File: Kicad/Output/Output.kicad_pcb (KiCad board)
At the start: 2 copper layers, 13 parts, among them J1 Conn_01x02, J2 Conn_01x03

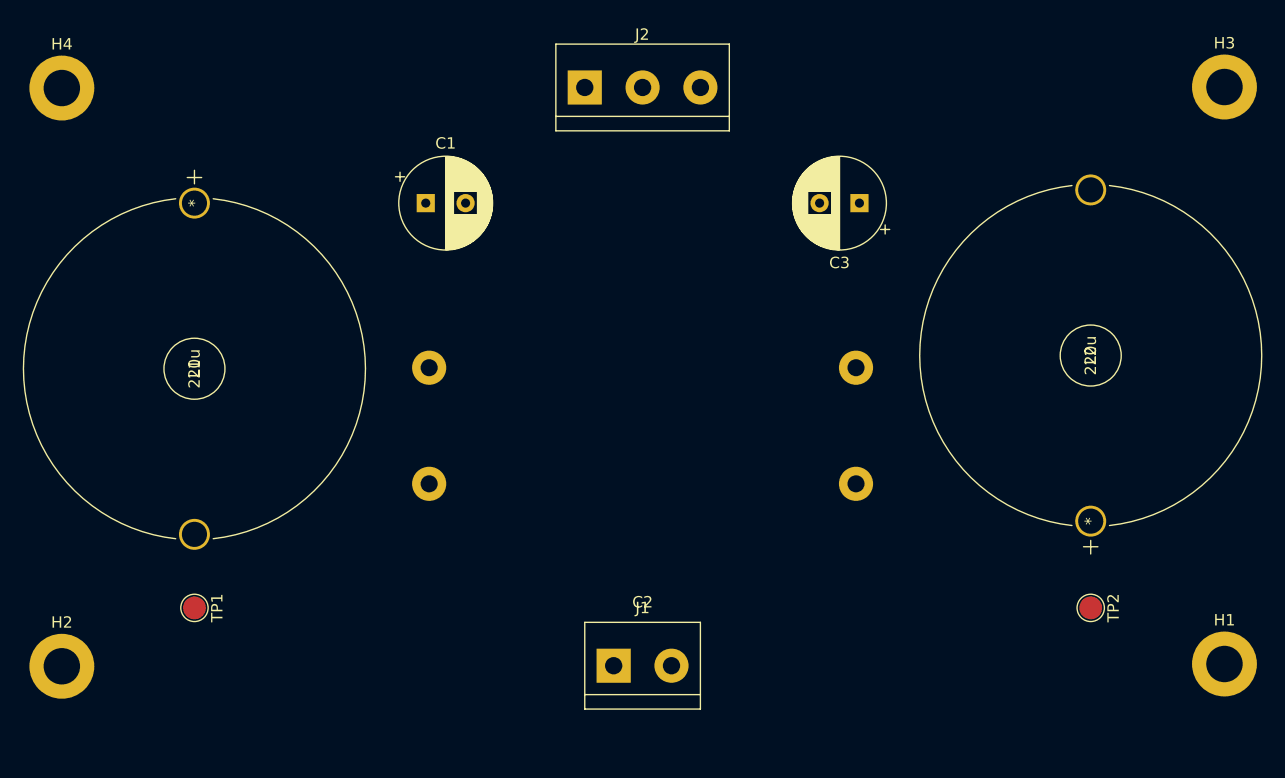
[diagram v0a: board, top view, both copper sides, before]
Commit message: OP Filter PCB Done
OP Filter PCB finished
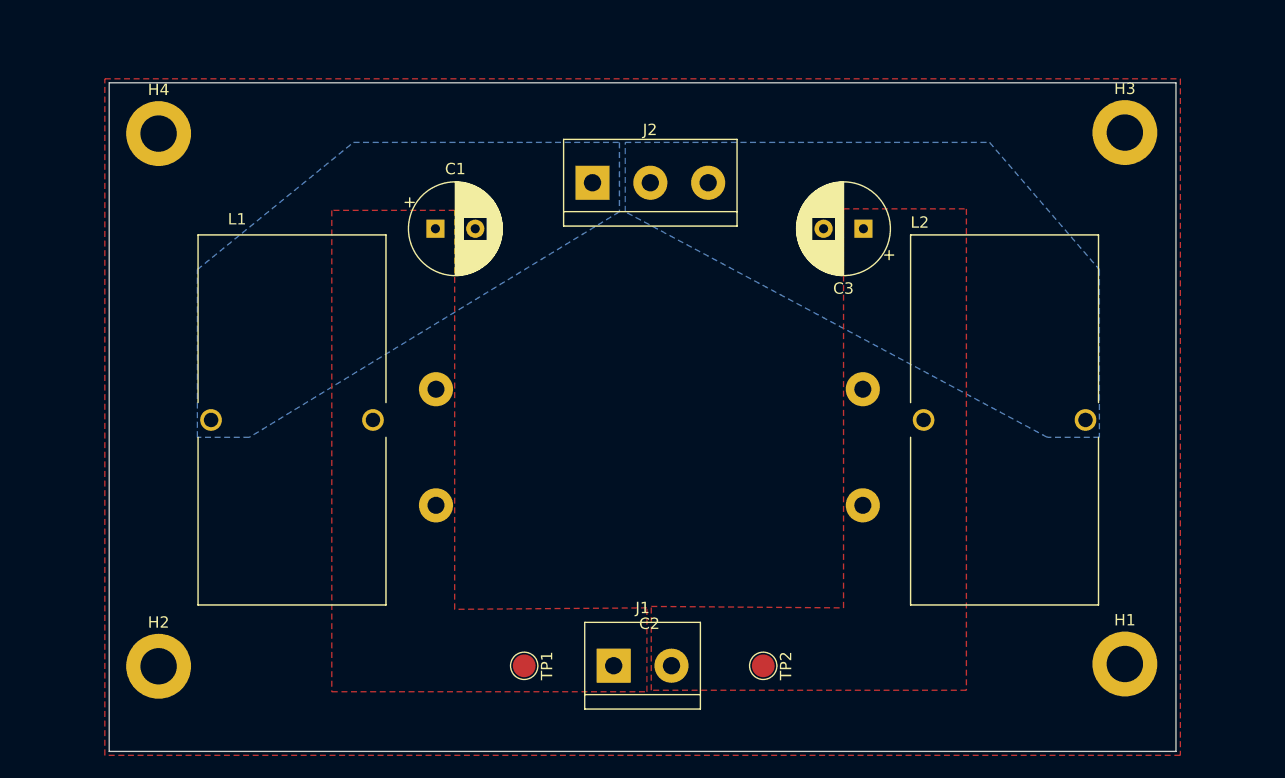
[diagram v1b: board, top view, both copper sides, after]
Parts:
- L1, L2: footprint 1422455C:1422455C -> OutputInductor:IND_HCTI-220-5.8
- moved TP1 29.4 mm to (142.0, 123.2)
- moved TP2 29.2 mm to (163.0, 123.2)
- moved L1 20.9 mm to (121.6, 101.6), turned to 0 degrees
- moved L2 11.7 mm to (184.2, 101.6), turned to 0 degrees
- moved H3 9.62 mm to (194.8, 76.3)
- moved H4 9.39 mm to (109.9, 76.4)
- moved H1 8.75 mm to (194.8, 123.0)
- moved H2 8.50 mm to (109.9, 123.2)
- moved J2 8.40 mm to (148.0, 80.8)
- moved C1 2.41 mm to (134.2, 84.8)
- moved C3 2.28 mm to (171.8, 84.8)
- moved C2 1.98 mm to (153.0, 120.0)
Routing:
- added copper zone on B.Cu, net /OutputFilter/SIG+
- added copper zone on B.Cu, net /OutputFilter/SIG-
- added copper zone on F.Cu, net /OutputFilter/SPEAKER+
- added copper zone on F.Cu, net /OutputFilter/SPEAKER-
- added copper zone on F.Cu, net GNDPWR
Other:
- board outline added: 93.7 x 58.7 mm
